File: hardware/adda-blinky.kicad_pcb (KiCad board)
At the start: 2 copper layers, 46.2 x 35.1 mm, 17 parts, among them J1 Conn_01x02, J2 Conn_01x02, J3 USB_B_Micro, J4 Conn_01x02, U1 ATtiny1616-S, U2 ATtiny1616-M, U3 AMS1117-3.3

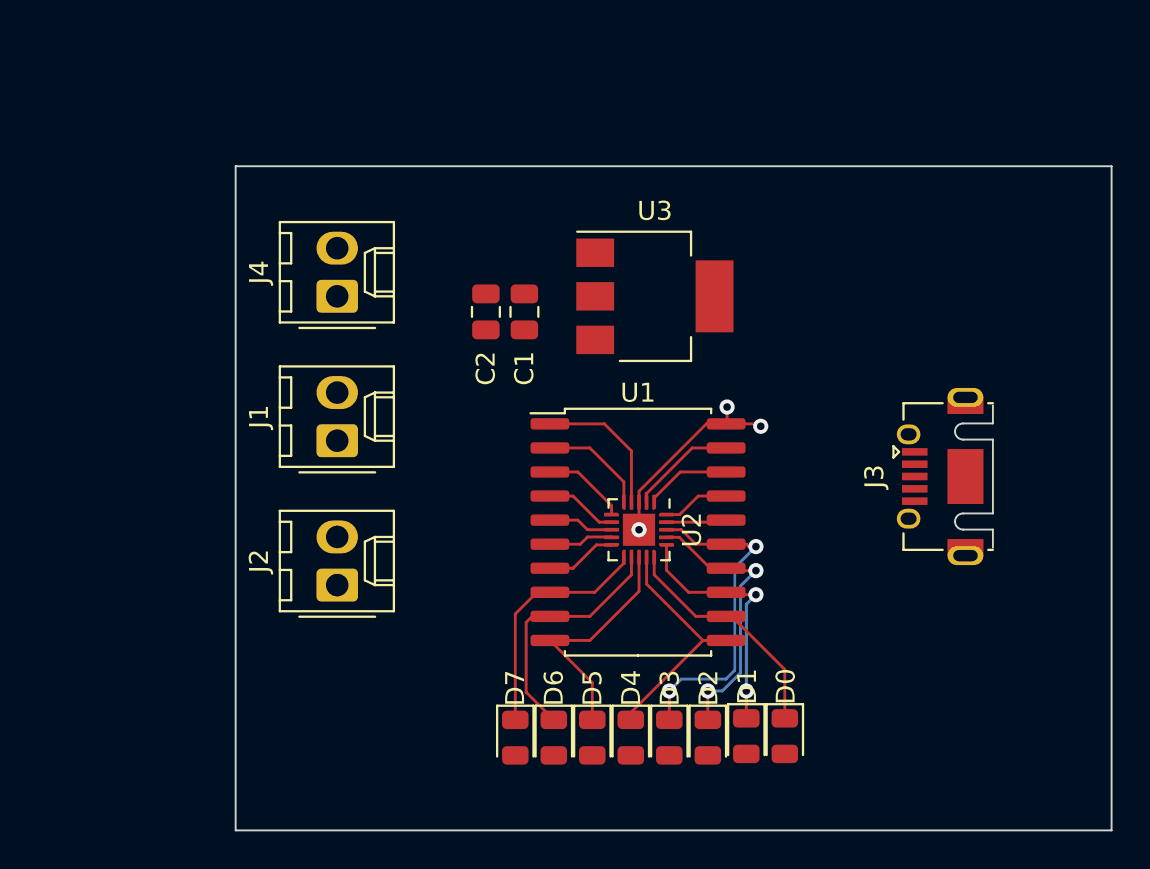
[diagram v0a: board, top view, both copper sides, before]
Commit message: First order
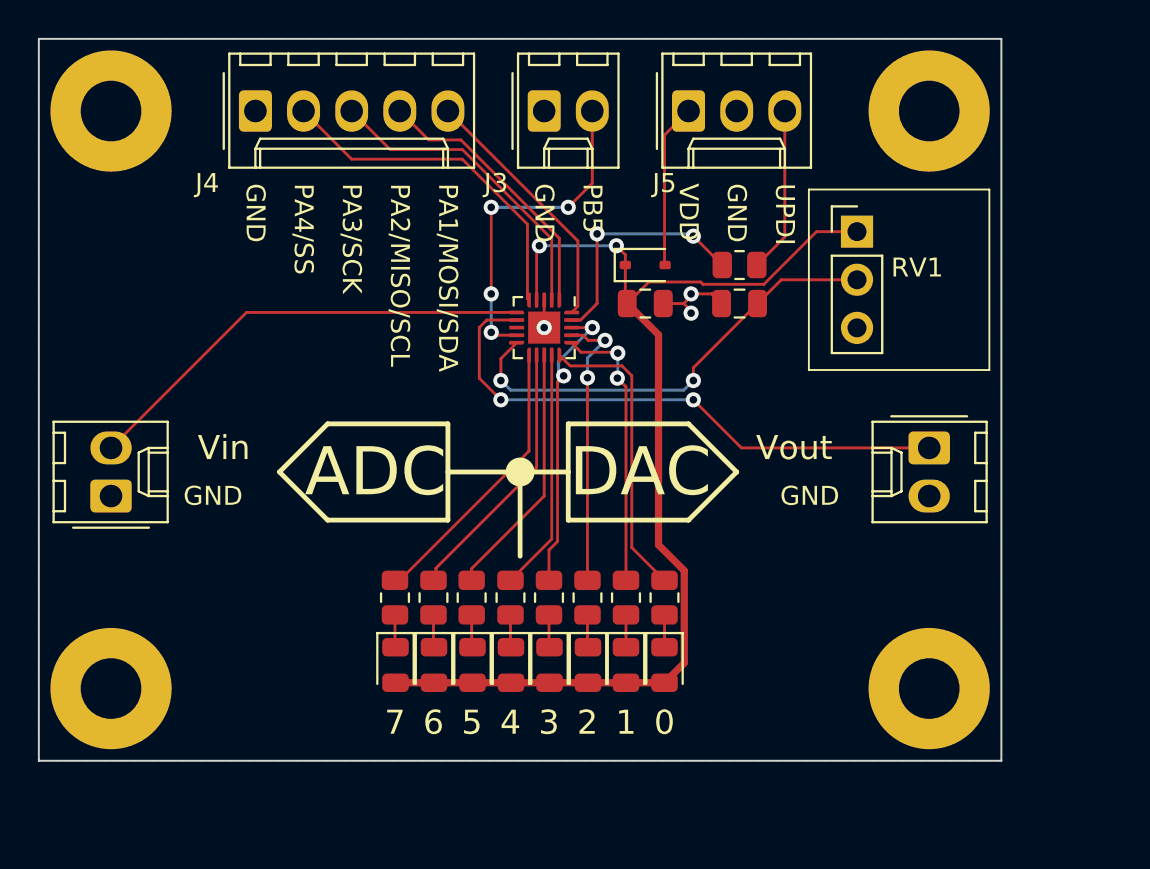
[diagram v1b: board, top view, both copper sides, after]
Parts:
- removed C2: 1u, Capacitor_SMD:C_0805_2012Metric
- removed U1: ATtiny1616-S, Package_SO:SOIC-20W_7.5x12.8mm_P1.27mm
- removed U3: AMS1117-3.3, Package_TO_SOT_SMD:SOT-223-3_TabPin2
- added C5: 1u, Capacitor_SMD:C_0805_2012Metric, F.Cu at (120.9, 52.1)
- added D10: 1N5819, Diode_SMD:D_SOD-323, F.Cu at (120.9, 50.0)
- added H1: MountingHole, MountingHole:MountingHole_3.2mm_M3_Pad, F.Cu at (92.7, 41.9)
- added H2: MountingHole, MountingHole:MountingHole_3.2mm_M3_Pad, F.Cu at (92.7, 72.4)
- added H3: MountingHole, MountingHole:MountingHole_3.2mm_M3_Pad, F.Cu at (135.9, 72.4)
- added H4: MountingHole, MountingHole:MountingHole_3.2mm_M3_Pad, F.Cu at (135.9, 41.9)
- added J5: PWR, Connector_Molex:Molex_KK-254_AE-6410-03A_1x03_P2.54mm_Vertical, F.Cu at (123.2, 41.9)
- added R0: 220, Resistor_SMD:R_0805_2012Metric, F.Cu at (121.9, 67.6)
- added R1: 220, Resistor_SMD:R_0805_2012Metric, F.Cu at (119.9, 67.6)
- added R2: 220, Resistor_SMD:R_0805_2012Metric, F.Cu at (117.9, 67.6)
- added R3: 220, Resistor_SMD:R_0805_2012Metric, F.Cu at (115.8, 67.6)
- added R4: 220, Resistor_SMD:R_0805_2012Metric, F.Cu at (113.8, 67.6)
- added R5: 220, Resistor_SMD:R_0805_2012Metric, F.Cu at (111.7, 67.6)
- added R6: 220, Resistor_SMD:R_0805_2012Metric, F.Cu at (109.7, 67.6)
- added R7: 220, Resistor_SMD:R_0805_2012Metric, F.Cu at (107.7, 67.6)
- added R8: 220, Resistor_SMD:R_0805_2012Metric, F.Cu at (125.9, 50.0)
- added RV1: R_Potentiometer, Connector_PinHeader_2.54mm:PinHeader_1x03_P2.54mm_Vertical, F.Cu at (132.1, 48.3)
- J1: value Conn_01x02 -> AIN
- J2: value Conn_01x02 -> AOUT
- J3: value USB_B_Micro -> PB5; footprint Connector_USB:USB_Micro-AB_Molex_47590-0001 -> Connector_Molex:Molex_KK-254_AE-6410-02A_1x02_P2.54mm_Vertical
- J4: value Conn_01x02 -> COMM; footprint Connector_Molex:Molex_KK-254_AE-6410-02A_1x02_P2.54mm_Vertical -> Connector_Molex:Molex_KK-254_AE-6410-05A_1x05_P2.54mm_Vertical
- moved J2 32.1 mm to (135.9, 59.7), turned to -90 degrees
- moved J3 29.4 mm to (115.6, 41.9), turned to 0 degrees
- moved J1 12.3 mm to (92.7, 62.2)
- moved U2 11.8 mm to (115.6, 53.3)
- moved C1 11.4 mm to (125.9, 52.1), turned to 180 degrees
- moved J4 10.7 mm to (100.3, 41.9), turned to 0 degrees
- moved D2 7.39 mm to (117.9, 71.1)
- moved D3 7.39 mm to (115.9, 71.1)
- moved D6 7.39 mm to (109.8, 71.1)
- moved D7 7.39 mm to (107.7, 71.1)
- moved D4 7.39 mm to (113.8, 71.1)
- moved D5 7.39 mm to (111.8, 71.1)
- moved D0 7.38 mm to (121.9, 71.1)
- moved D1 7.38 mm to (119.9, 71.1)
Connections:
- C1 pad 1: +3.3V -> /PB4
- D0 pad 1: /PC0 -> Net-(D0-K)
- D0 pad 2: +3.3V -> +5V
- D1 pad 1: /PC1 -> Net-(D1-K)
- D1 pad 2: +3.3V -> +5V
- D2 pad 1: /PC2 -> Net-(D2-K)
- D2 pad 2: +3.3V -> +5V
- D3 pad 1: /PC3 -> Net-(D3-K)
- D3 pad 2: +3.3V -> +5V
- D4 pad 1: /PB0 -> Net-(D4-K)
- D4 pad 2: +3.3V -> +5V
- D5 pad 1: /PB1 -> Net-(D5-K)
- D5 pad 2: +3.3V -> +5V
- D6 pad 1: /PB2 -> Net-(D6-K)
- D6 pad 2: +3.3V -> +5V
- D7 pad 1: /PB3 -> Net-(D7-K)
- D7 pad 2: +3.3V -> +5V
- J1 pad 1: /PA5/AIN5 -> GND
- J1 pad 2: GND -> /PA5/AIN5
- J3 pad 1: Net-(D8-A) -> GND
- J3 pad 2: unconnected-(J3-D--Pad2) -> /PB5
- J4 pad 1: +VDC -> GND
- J4 pad 2: GND -> /PA4/SS
- U2 pad 4: +3.3V -> +5V
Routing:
- net +5V: track 0.00 -> 60.0 mm, vias 0 -> 2
- net /PA6/OUT: track 3.82 -> 30.1 mm, vias 0 -> 2
- net /PB4: track 3.76 -> 24.2 mm, vias 0 -> 2
- net /PA5/AIN5: track 4.46 -> 24.4 mm
- net /PB5: track 3.42 -> 17.7 mm, vias 0 -> 4
- net /PA4/SS: track 5.72 -> 18.3 mm
- net /PA3/SCK: track 5.69 -> 16.6 mm
- net /PA1/MOSI/SDA: track 3.55 -> 13.6 mm
- net /PA2/MISO/SCL: track 4.59 -> 14.5 mm
- net /~{RESET}: track 3.19 -> 12.7 mm, vias 0 -> 2
- net /UPDI: track 0.00 -> 8.74 mm
- net Net-(D10-A): track 0.00 -> 8.65 mm
- net +3.3V: track 7.77 -> 0.00 mm
- net GND: track 10.9 -> 5.69 mm
- net /PA7: track 3.46 -> 0.00 mm
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- added copper zone on B.Cu, net GND
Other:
- board size 46.2 x 35.1 mm -> 50.8 x 38.1 mm
- board text added: "0"
- board text added: "1"
- board text added: "2"
- board text added: "3"
- board text added: "4"
- board text added: "5"
- board text added: "6"
- board text added: "7"
- board text added: "ADC"
- board text added: "DAC"
- board text added: "GND"
- board text added: "PA1/MOSI/SDA"
- board text added: "PA2/MISO/SCL"
- board text added: "PA3/SCK"
- board text added: "PA4/SS"
- board text added: "PB5"
- board text added: "UPDI"
- board text added: "VDD"
- board text added: "Vin"
- board text added: "Vout"
